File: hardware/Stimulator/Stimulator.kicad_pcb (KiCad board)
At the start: 2 copper layers, 101.6 x 32.4 mm, 152 parts, among them P1 CONN_1, P10 CONN_1, P11 CONN_1, P12 CONN_1, P13 CONN_1, P14 CONN_1, P15 CONN_10, P16 CONN_1, P17 CONN_1, P18 CONN_1, P19 CONN_10X2, P2 CONN_1, P20 CONN_1, P21 CONN_1, P22 CONN_1, P23 TEST, P24 CONN_10, P25 TEST, P26 CONN_1, P27 CONN_1, P28 CONN_1, P29 CONN_1, P3 CONN_1, P30 CONN_1, P31 CONN_1, P32 CONN_1, P33 CONN_1, P34 CONN_1, P35 CONN_1, P36 CONN_1, P37 CONN_1, P38 CONN_1, P39 CONN_1, P4 CONN_1, P40 TEST, P41 CONN_1, P42 CONN_1, P43 CONN_1, P44 CONN_1, P45 CONN_1, P46 CONN_1, P47 CONN_1, P48 CONN_1, P49 CONN_1, P5 CONN_1, P50 CONN_1, P51 CONN_1, P52 CONN_1, P53 CONN_1, P54 CONN_1, P55 CONN_1, P56 CONN_1, P57 CONN_1, P58 CONN_1, P59 CONN_1, P6 CONN_1, P60 CONN_1, P61 CONN_1, P62 CONN_1, P63 CONN_1, P64 CONN_10, P65 CONN_1, P66 CONN_1, P67 CONN_1, P68 CONN_1, P69 CONN_1, P7 TEST, P70 CONN_10X2, P71 CONN_1, P72 CONN_1, P73 CONN_1, P74 CONN_1, P75 CONN_10, P76 CONN_1, P77 CONN_1, P78 TEST, P79 TEST, P8 TEST, P80 DIL16, P81 DIL16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

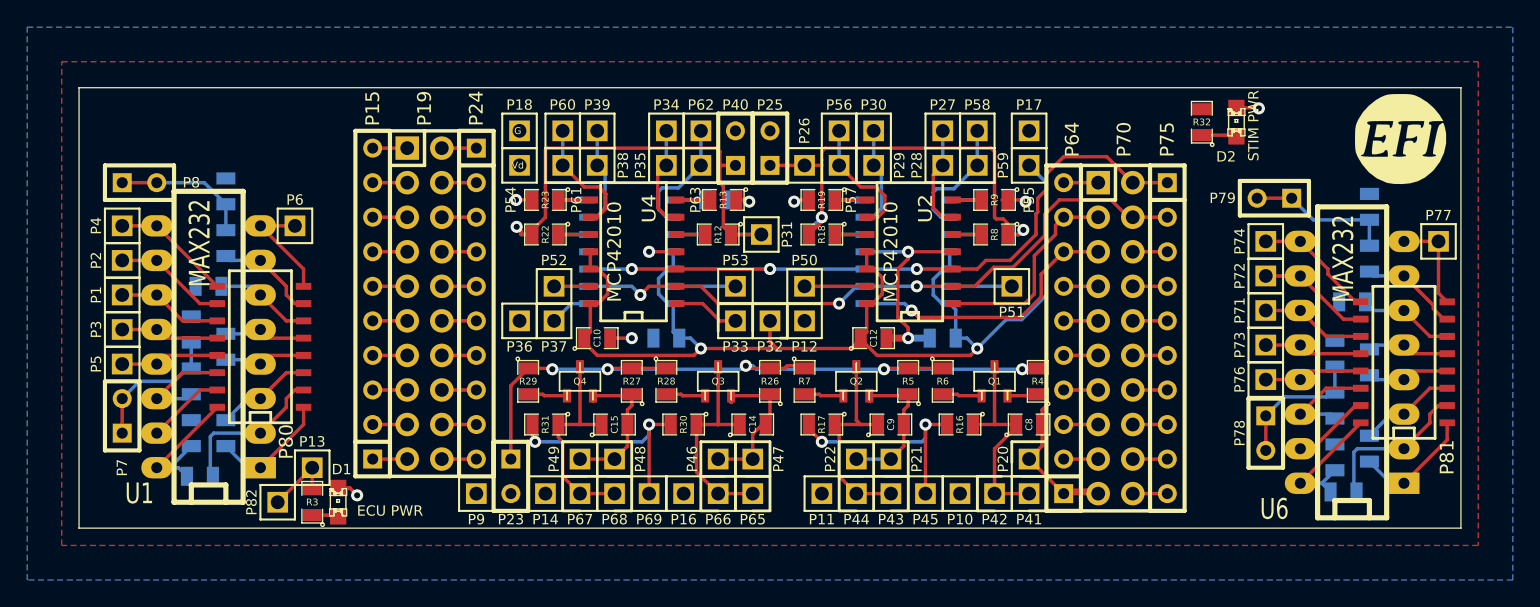
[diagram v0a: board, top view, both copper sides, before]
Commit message: update pcb files
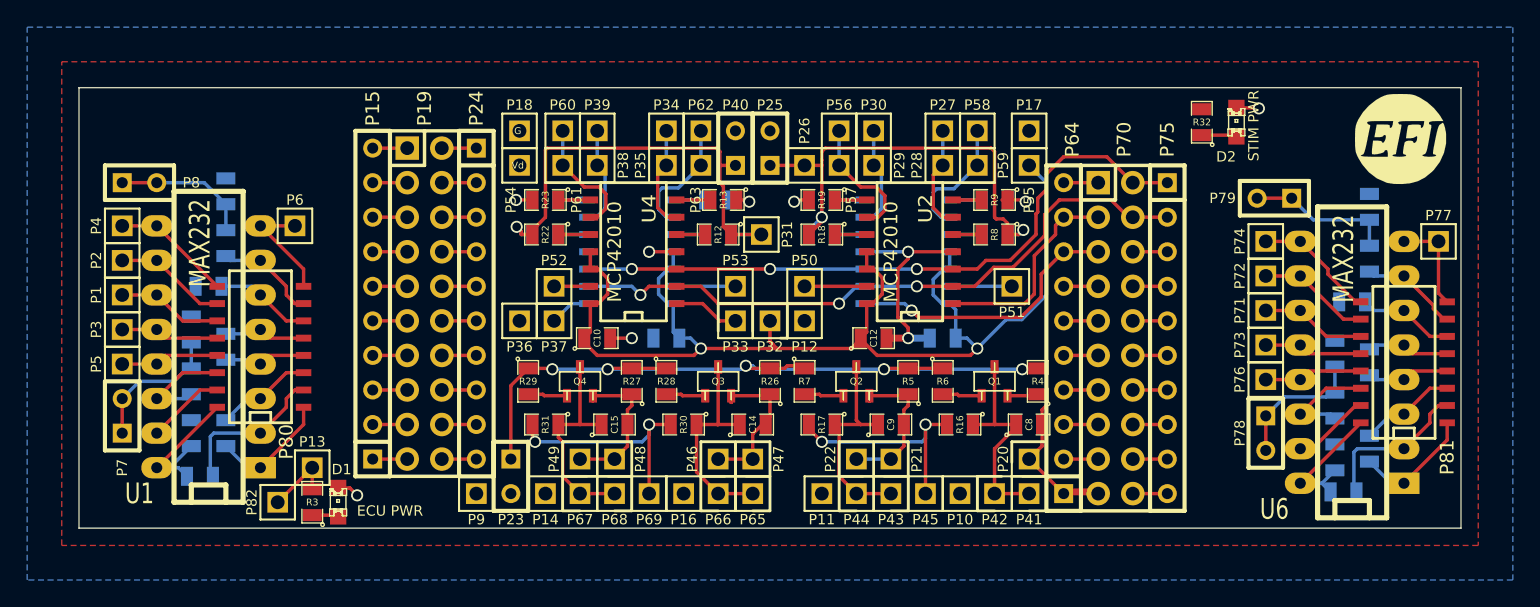
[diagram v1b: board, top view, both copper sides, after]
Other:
- net class Default removed
- net class Power removed
